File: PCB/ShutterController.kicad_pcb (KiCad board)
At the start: 2 copper layers, 73.7 x 53.3 mm, 32 parts, among them J1 Screw_Terminal_01x03, J2 Screw_Terminal_01x02, Q1 TS13003, Q2 TS13003, Q3 TS13003, Q4 TS13003, Q5 TS13003, Q6 TS13003, Q7 TS13003, U1 LM7805_TO220, U2 PIC16(L)F627A-I/P

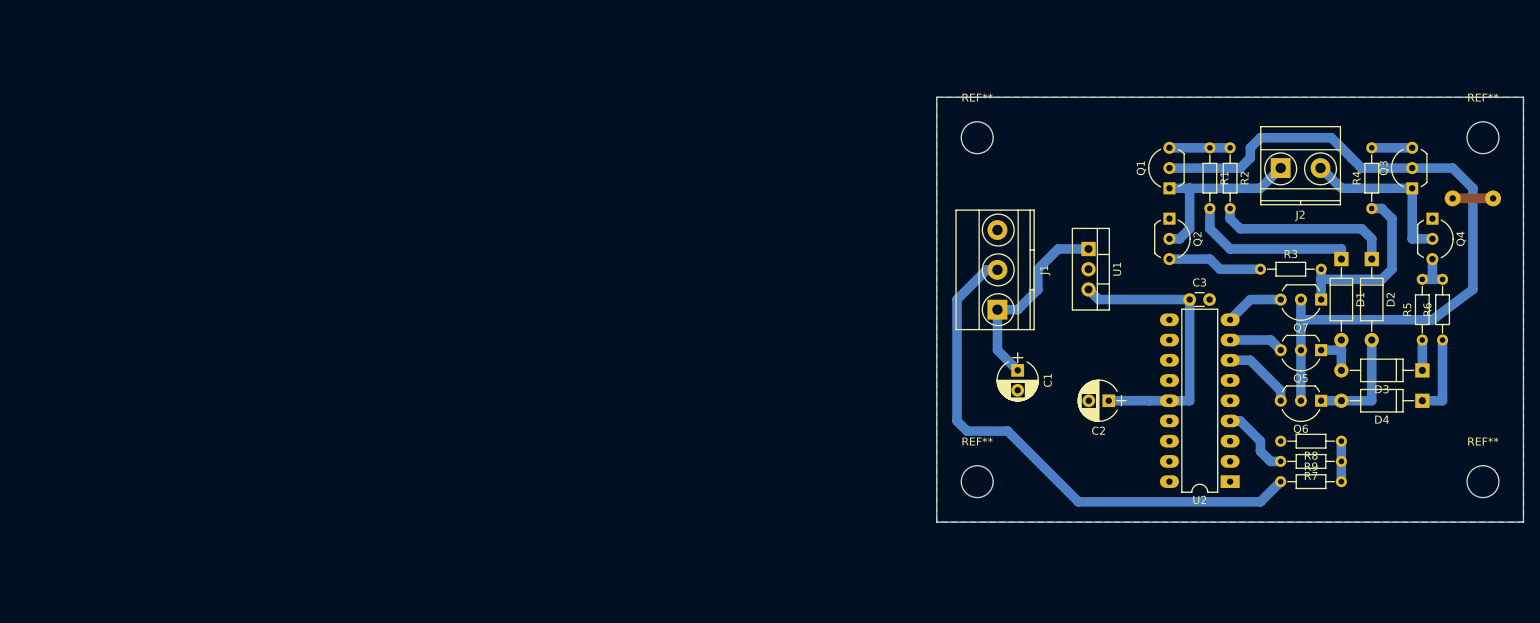
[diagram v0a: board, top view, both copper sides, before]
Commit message: Update
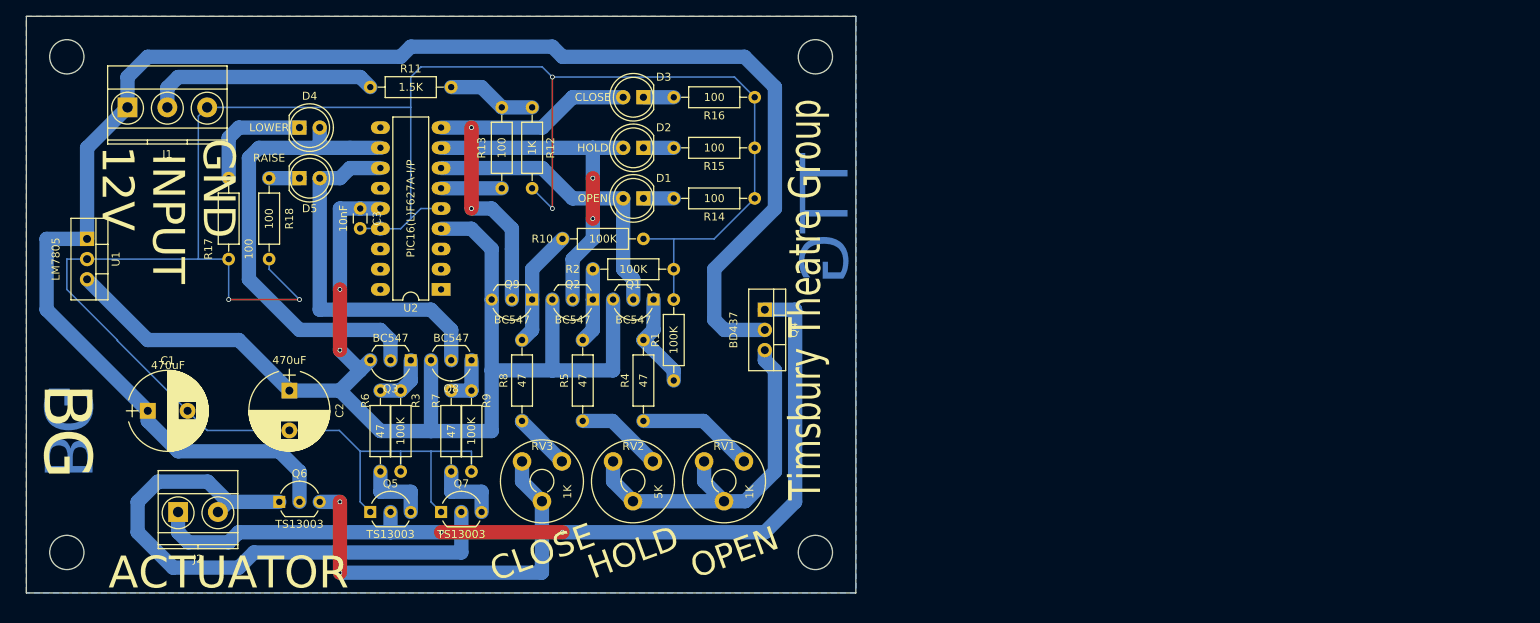
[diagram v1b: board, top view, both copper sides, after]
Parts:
- removed the REF** at (213.4, 44.5)
- removed the REF** at (201.9, 31.8)
- removed the REF** at (138.4, 74.9)
- removed the REF** at (201.9, 74.9)
- removed the REF** at (138.4, 31.8)
- added D5: RAISE, LEDs:LED_D5.0mm, F.Cu at (53.3, 36.8)
- added Q8: BC547, TO_SOT_Packages_THT:TO-92_Inline_Wide, F.Cu at (74.9, 59.7)
- added Q9: BC547, TO_SOT_Packages_THT:TO-92_Inline_Wide, F.Cu at (82.5, 52.1)
- added R10: 100K, Resistors_THT:R_Axial_DIN0207_L6.3mm_D2.5mm_P10.16mm_Horizontal, F.Cu at (96.5, 44.5)
- added R11: 1.5K, Resistors_THT:R_Axial_DIN0207_L6.3mm_D2.5mm_P10.16mm_Horizontal, F.Cu at (62.2, 25.4)
- added R12: 1K, Resistors_THT:R_Axial_DIN0207_L6.3mm_D2.5mm_P10.16mm_Horizontal, F.Cu at (82.5, 27.9)
- added R13: 100, Resistors_THT:R_Axial_DIN0207_L6.3mm_D2.5mm_P10.16mm_Horizontal, F.Cu at (78.7, 27.9)
- added R14: 100, Resistors_THT:R_Axial_DIN0207_L6.3mm_D2.5mm_P10.16mm_Horizontal, F.Cu at (110.5, 39.4)
- added R15: 100, Resistors_THT:R_Axial_DIN0207_L6.3mm_D2.5mm_P10.16mm_Horizontal, F.Cu at (110.5, 33.0)
- added R16: 100, Resistors_THT:R_Axial_DIN0207_L6.3mm_D2.5mm_P10.16mm_Horizontal, F.Cu at (110.5, 26.7)
- added R17: 100, Resistors_THT:R_Axial_DIN0207_L6.3mm_D2.5mm_P10.16mm_Horizontal, F.Cu at (44.5, 47.0)
- added R18: 100, Resistors_THT:R_Axial_DIN0207_L6.3mm_D2.5mm_P10.16mm_Horizontal, F.Cu at (49.5, 47.0)
- added REF**: MountingHole_4.3mm_M4, Mounting_Holes:MountingHole_4.3mm_M4, F.Cu at (118.1, 21.6)
- added REF**: MountingHole_4.3mm_M4, Mounting_Holes:MountingHole_4.3mm_M4, F.Cu at (24.1, 21.6)
- added REF**: MountingHole_4.3mm_M4, Mounting_Holes:MountingHole_4.3mm_M4, F.Cu at (24.1, 83.8)
- added REF**: MountingHole_4.3mm_M4, Mounting_Holes:MountingHole_4.3mm_M4, F.Cu at (118.1, 83.8)
- added RV1: 1K, Potentiometers:Potentiometer_Trimmer_Piher_PT-10v5_Horizontal_Px5.0mm_Py5.0mm, F.Cu at (104.1, 72.4)
- added RV2: 5K, Potentiometers:Potentiometer_Trimmer_Piher_PT-10v5_Horizontal_Px5.0mm_Py5.0mm, F.Cu at (92.7, 72.4)
- added RV3: 1K, Potentiometers:Potentiometer_Trimmer_Piher_PT-10v5_Horizontal_Px5.0mm_Py5.0mm, F.Cu at (81.3, 72.4)
- C1, C2: footprint Capacitors_THT:CP_Radial_D5.0mm_P2.50mm -> Capacitors_THT:CP_Radial_D10.0mm_P5.00mm
- D1: value D -> OPEN; footprint Diodes_THT:D_A-405_P10.16mm_Horizontal -> LEDs:LED_D5.0mm
- D2: value D -> HOLD; footprint Diodes_THT:D_A-405_P10.16mm_Horizontal -> LEDs:LED_D5.0mm
- D3: value D -> CLOSE; footprint Diodes_THT:D_A-405_P10.16mm_Horizontal -> LEDs:LED_D5.0mm
- D4: value D -> LOWER; footprint Diodes_THT:D_A-405_P10.16mm_Horizontal -> LEDs:LED_D5.0mm
- Q1, Q2, Q3: value TS13003 -> BC547
- Q4: value TS13003 -> BD437; footprint TO_SOT_Packages_THT:TO-92_Inline_Wide -> TO_SOT_Packages_THT:TO-220-3_Vertical
- R1, R2: value 100 -> 100K; footprint Resistors_THT:R_Axial_DIN0204_L3.6mm_D1.6mm_P7.62mm_Horizontal -> Resistors_THT:R_Axial_DIN0207_L6.3mm_D2.5mm_P10.16mm_Horizontal
- R3, R9: value 1K -> 100K; footprint Resistors_THT:R_Axial_DIN0204_L3.6mm_D1.6mm_P7.62mm_Horizontal -> Resistors_THT:R_Axial_DIN0207_L6.3mm_D2.5mm_P10.16mm_Horizontal
- R4, R7: value 100 -> 47; footprint Resistors_THT:R_Axial_DIN0204_L3.6mm_D1.6mm_P7.62mm_Horizontal -> Resistors_THT:R_Axial_DIN0207_L6.3mm_D2.5mm_P10.16mm_Horizontal
- R5: value 810 -> 47; footprint Resistors_THT:R_Axial_DIN0204_L3.6mm_D1.6mm_P7.62mm_Horizontal -> Resistors_THT:R_Axial_DIN0207_L6.3mm_D2.5mm_P10.16mm_Horizontal
- R6: value 120 -> 47; footprint Resistors_THT:R_Axial_DIN0204_L3.6mm_D1.6mm_P7.62mm_Horizontal -> Resistors_THT:R_Axial_DIN0207_L6.3mm_D2.5mm_P10.16mm_Horizontal
- R8: value 1K -> 47; footprint Resistors_THT:R_Axial_DIN0204_L3.6mm_D1.6mm_P7.62mm_Horizontal -> Resistors_THT:R_Axial_DIN0207_L6.3mm_D2.5mm_P10.16mm_Horizontal
- U1: value LM7805_TO220 -> LM7805
- moved D4 145.1 mm to (53.3, 30.5), turned to 0 degrees
- moved J2 145.0 mm to (38.1, 78.7)
- moved R6 134.4 mm to (63.5, 73.7)
- moved Q6 131.4 mm to (50.8, 77.5), turned to 0 degrees
- moved Q3 127.6 mm to (67.3, 59.7), turned to 180 degrees
- moved U1 125.7 mm to (26.7, 44.5)
- moved Q5 121.1 mm to (62.2, 78.7), turned to 0 degrees
- moved Q7 113.7 mm to (71.1, 78.7), turned to 0 degrees
- moved J1 112.1 mm to (31.8, 27.9), turned to 0 degrees
- moved R7 112.1 mm to (72.4, 63.5), turned to 270 degrees
- moved C1 109.3 mm to (34.3, 66.0), turned to 0 degrees
- moved R3 109.0 mm to (66.0, 63.5), turned to 270 degrees
- moved R5 105.9 mm to (88.9, 67.3)
- moved C3 104.8 mm to (61.0, 40.6), turned to 270 degrees
- moved D3 103.6 mm to (96.5, 26.7)
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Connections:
- C1 pad 1: Net-(C1-Pad1) -> 12V
- C2 pad 1: VCC -> VDD
- C3 pad 1: VCC -> VDD
- D1 pad 2: M_HOLD -> OPEN
- D2 pad 2: M_OPEN -> HOLD
- D3 pad 2: M_HOLD -> CLOSE
- D4 pad 2: M_OPEN -> LOWER
- J1 pad 1: Net-(C1-Pad1) -> 12V
- Q1 pad 1: Net-(J2-Pad1) -> Net-(Q1-Pad1)
- Q1 pad 2: VCC -> OPEN
- Q1 pad 3: Net-(Q1-Pad3) -> VDD
- Q2 pad 1: GND -> Net-(Q2-Pad1)
- Q2 pad 2: Net-(J2-Pad1) -> HOLD
- Q2 pad 3: Net-(Q2-Pad3) -> VDD
- Q3 pad 1: Net-(J2-Pad2) -> Net-(Q3-Pad1)
- Q3 pad 2: VCC -> LOWER
- Q3 pad 3: Net-(Q3-Pad3) -> VDD
- Q4 pad 1: GND -> Net-(J2-Pad1)
- Q4 pad 2: Net-(J2-Pad2) -> 12V
- Q5 pad 1: M_HOLD -> GND
- Q5 pad 2: VCC -> Net-(J2-Pad1)
- Q5 pad 3: HOLD -> Net-(Q5-Pad3)
- Q6 pad 1: M_OPEN -> Net-(J2-Pad2)
- Q6 pad 2: VCC -> 12V
- Q6 pad 3: OPEN -> Net-(Q6-Pad3)
- Q7 pad 1: M_CLOSE -> GND
- Q7 pad 2: VCC -> Net-(J2-Pad2)
- Q7 pad 3: CLOSE -> Net-(Q7-Pad3)
- R1 pad 1: Net-(Q1-Pad3) -> Net-(Q1-Pad1)
- R1 pad 2: Net-(D1-Pad1) -> GND
- R2 pad 1: Net-(Q1-Pad3) -> Net-(Q2-Pad1)
- R2 pad 2: Net-(D2-Pad1) -> GND
- R3 pad 1: Net-(Q2-Pad3) -> Net-(Q3-Pad1)
- R3 pad 2: M_CLOSE -> GND
- R4 pad 1: M_CLOSE -> Net-(R4-Pad1)
- R4 pad 2: Net-(Q3-Pad3) -> Net-(Q1-Pad1)
- R5 pad 1: Net-(D3-Pad1) -> Net-(R5-Pad1)
- R5 pad 2: Net-(Q4-Pad3) -> Net-(Q2-Pad1)
- R6 pad 1: Net-(D4-Pad1) -> Net-(Q5-Pad3)
- R6 pad 2: Net-(Q4-Pad3) -> Net-(Q3-Pad1)
- R7 pad 1: Net-(R7-Pad1) -> Net-(Q8-Pad1)
- R7 pad 2: Net-(R7-Pad2) -> Net-(Q7-Pad3)
- R8 pad 1: Net-(R7-Pad1) -> Net-(R8-Pad1)
- R8 pad 2: GND -> Net-(Q9-Pad1)
- R9 pad 1: INPUT -> GND
- R9 pad 2: Net-(R7-Pad1) -> Net-(Q8-Pad1)
- U1 pad 1: Net-(C1-Pad1) -> 12V
- U1 pad 3: VCC -> VDD
- U2 pad 11: Net-(U2-Pad11) -> LOWER
- U2 pad 12: Net-(U2-Pad12) -> RAISE
- U2 pad 14: VCC -> VDD
- U2 pad 15: Net-(U2-Pad15) -> GND
- U2 pad 4: Net-(R7-Pad2) -> VDD
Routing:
- net GND: track 5.08 -> 301.3 mm, vias 0 -> 4
- net 12V: track 0.00 -> 205.3 mm
- net VDD: track 0.00 -> 162.7 mm, vias 0 -> 2
- net VCC: track 127.4 -> 0.00 mm
- net Net-(J2-Pad1): track 23.2 -> 113.1 mm, vias 0 -> 2
- net LOWER: track 0.00 -> 58.3 mm
- net Net-(J2-Pad2): track 21.5 -> 73.8 mm
- net Net-(Q6-Pad3): track 0.00 -> 51.8 mm, vias 0 -> 2
- net RAISE: track 0.00 -> 46.0 mm
- net Net-(Q4-Pad3): track 5.08 -> 47.3 mm
- net CLOSE: track 7.40 -> 49.6 mm, vias 0 -> 2
- net INPUT: track 67.8 -> 29.0 mm
- net HOLD: track 6.88 -> 43.0 mm, vias 0 -> 2
- net OPEN: track 9.20 -> 37.7 mm
- net Net-(C1-Pad1): track 24.7 -> 0.00 mm
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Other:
- board size 73.7 x 53.3 mm -> 104.1 x 72.4 mm
- net class Default: clearance 0.4 -> 0.2; trace_width 1.2 -> 1.8
- net class GND added: clearance 0.2, trace_width 0.2, via_dia 0.6, via_drill 0.4
- rule pad_to_mask_clearance: 0.2 -> 0
- rule trace_clearance: 0.4 -> 0.2
- board text added: "12V"
- board text added: "ACTUATOR"
- board text added: "BG"
- board text added: "CLOSE"
- board text added: "GND"
- board text added: "HOLD"
- board text added: "INPUT"
- board text added: "OPEN"
- board text added: "TTG"
- board text added: "Timsbury Theatre Group"
